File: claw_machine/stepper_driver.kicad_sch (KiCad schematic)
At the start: 2 parts, among them J6 Screw_Terminal_01x04

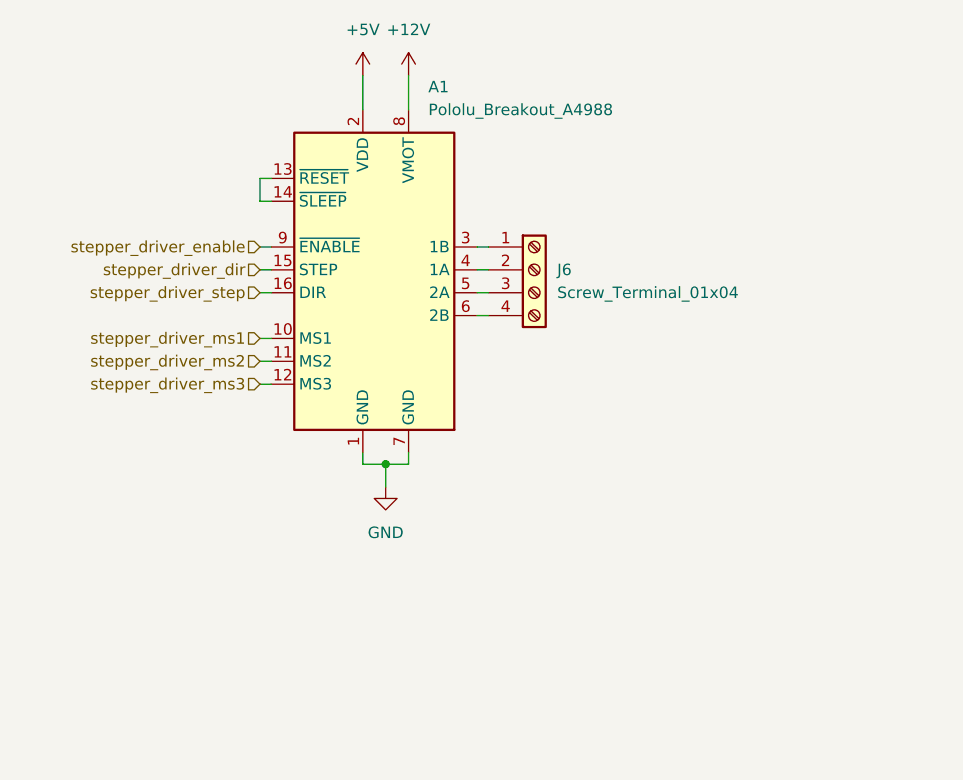
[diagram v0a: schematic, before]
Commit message: change folder stuff & update gen pwr
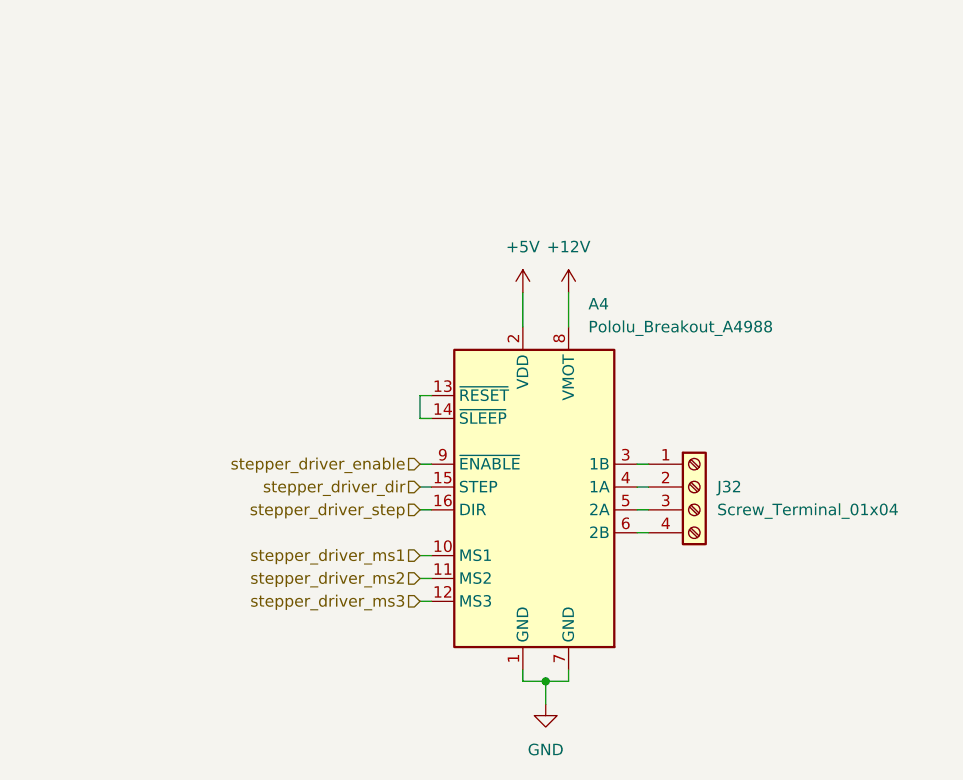
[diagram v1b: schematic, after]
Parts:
- removed A1: Pololu_Breakout_A4988, Module:Pololu_Breakout-16_15.2x20.3mm, symbol Driver_Motor:Pololu_Breakout_A4988
- removed J6: Screw_Terminal_01x04, symbol Connector:Screw_Terminal_01x04
- added A4: Pololu_Breakout_A4988, Module:Pololu_Breakout-16_15.2x20.3mm, symbol Driver_Motor:Pololu_Breakout_A4988
- added J32: Screw_Terminal_01x04, TerminalBlock:TerminalBlock_bornier-4_P5.08mm, symbol Connector:Screw_Terminal_01x04
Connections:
- net +12V: now also A4.8 (VMOT)
- net +5V: now also A4.2 (VDD)
- net GND: now also A4.1 (GND), A4.7 (GND)
- net stepper_driver_dir: now also A4.15 (STEP)
- net stepper_driver_enable: now also A4.9 (~{ENABLE})
- net stepper_driver_ms1: now also A4.10 (MS1)
- net stepper_driver_ms2: now also A4.11 (MS2)
- net stepper_driver_ms3: now also A4.12 (MS3)
- net stepper_driver_step: now also A4.16 (DIR)
- new net: A4.3 (1B), J32.1 (Pin_1)
- new net: A4.4 (1A), J32.2 (Pin_2)
- new net: A4.5 (2A), J32.3 (Pin_3)
- new net: A4.6 (2B), J32.4 (Pin_4)
- new net: A4.13 (~{RESET}), A4.14 (~{SLEEP})
